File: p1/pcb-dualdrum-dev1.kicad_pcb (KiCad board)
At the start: 2 copper layers, 48 x 109.2 mm, 156 parts, among them P1 CONN-02x05, U1 082, U2 082, U3 082, U4 082, U5 082, U6 082, U7 082, U8 082-NJM, U9 082

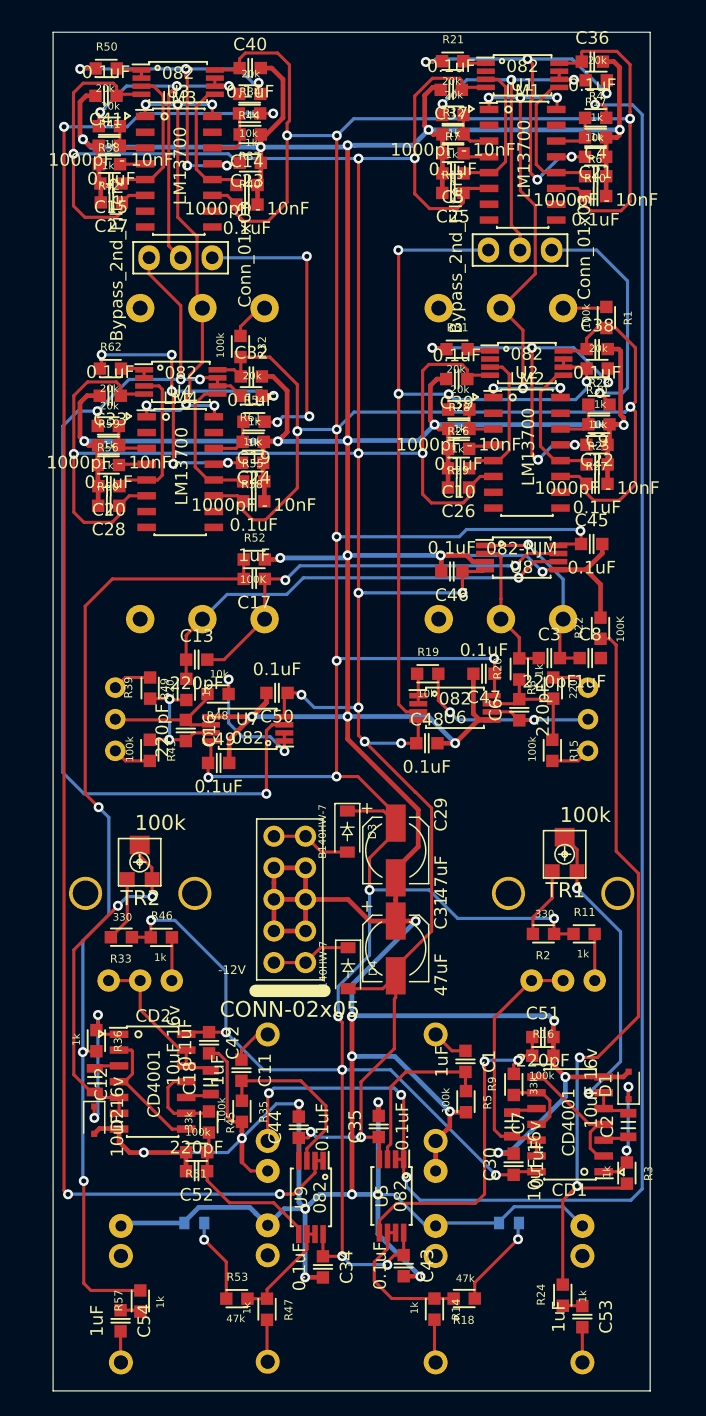
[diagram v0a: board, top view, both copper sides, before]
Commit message: drc cleared - checking for more mistakes
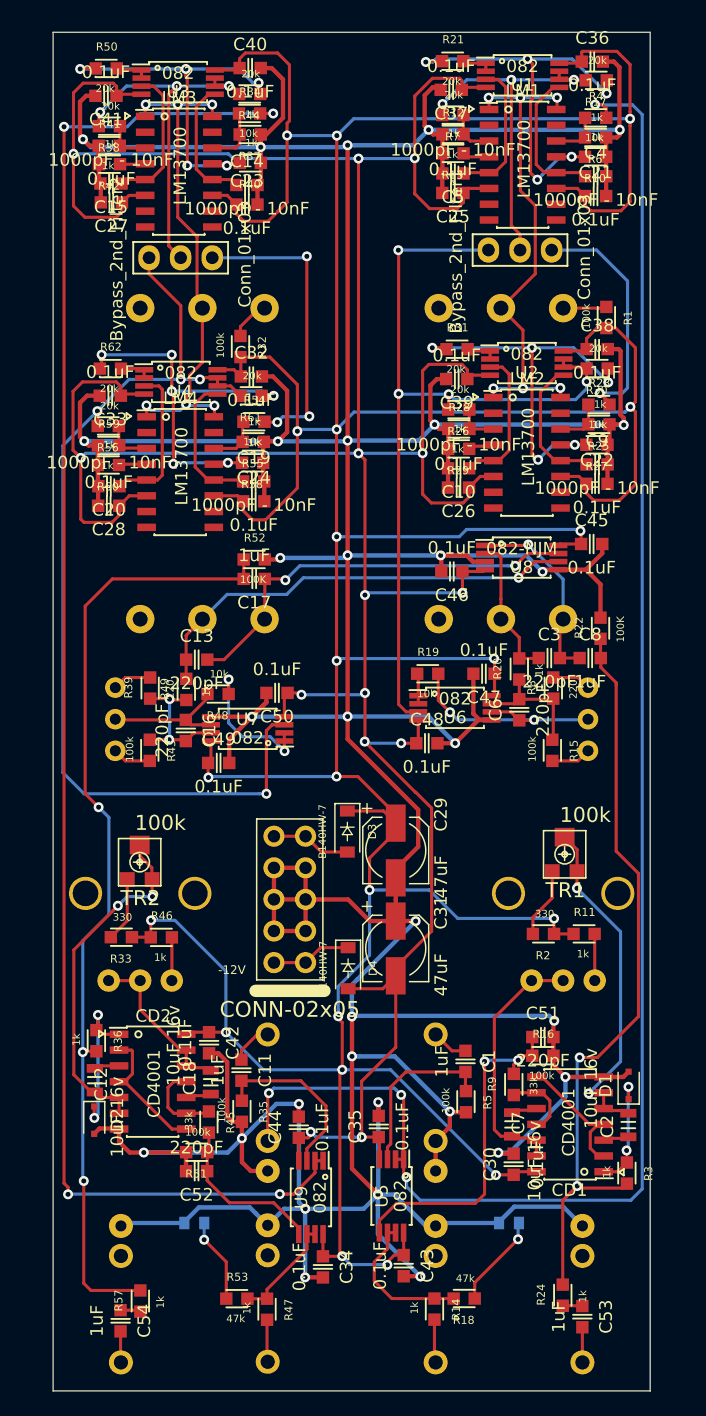
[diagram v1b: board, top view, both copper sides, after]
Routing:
- net Net-(Bypass_2nd_Filter2-Pad1): track 81.1 -> 80.1 mm
- net GND: track 546.9 -> 547.8 mm, vias 33 -> 32
- net Net-(R21-Pad1): track 1.88 -> 2.53 mm
- net Net-(R31-Pad1): track 1.86 -> 2.51 mm
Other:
- rule trace_min: 0.2 -> 0
